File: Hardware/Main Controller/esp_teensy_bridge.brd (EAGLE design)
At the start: 102.8 x 87.9 mm, 42 parts, among them IC1 BQ79600PWRQ1, Q1 SI7611DN-T1-GE3, Q2 SI7611DN-T1-GE3, Q3 SI7611DN-T1-GE3, Q4 SI7611DN-T1-GE3

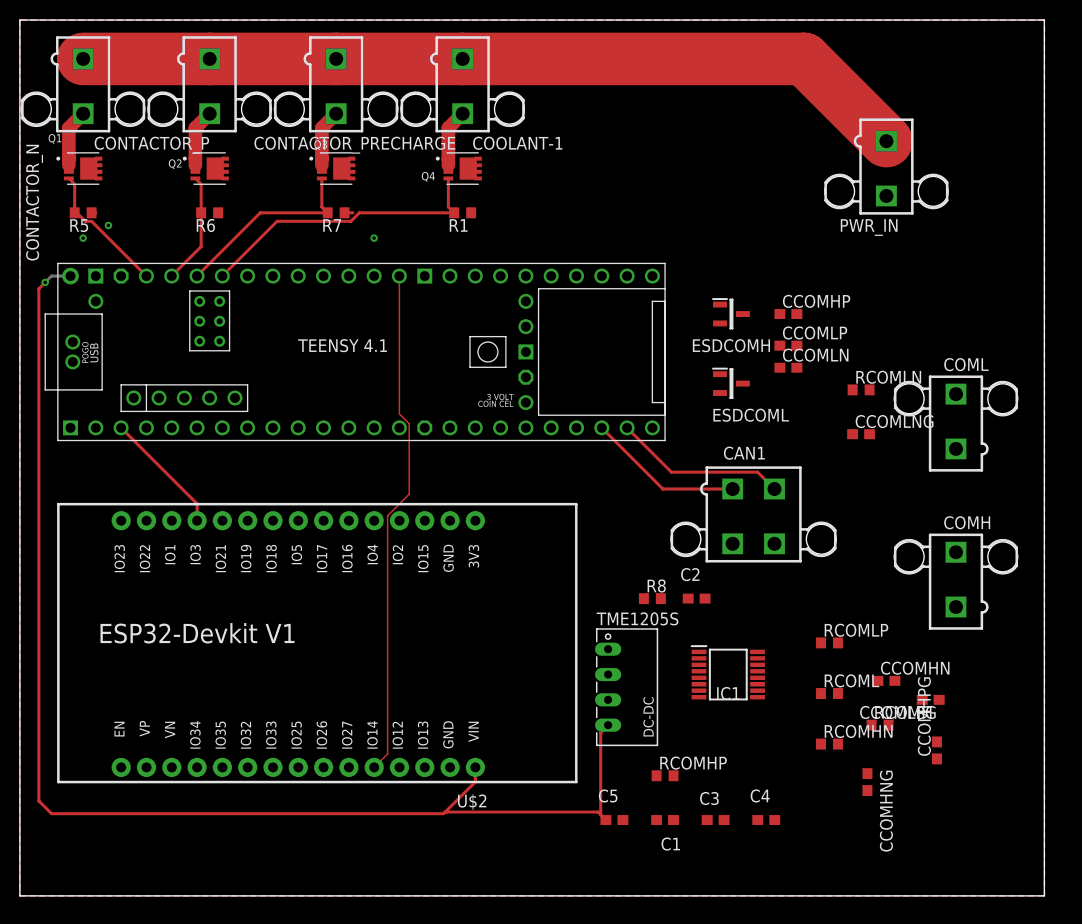
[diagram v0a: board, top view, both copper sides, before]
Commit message: connected some stuff
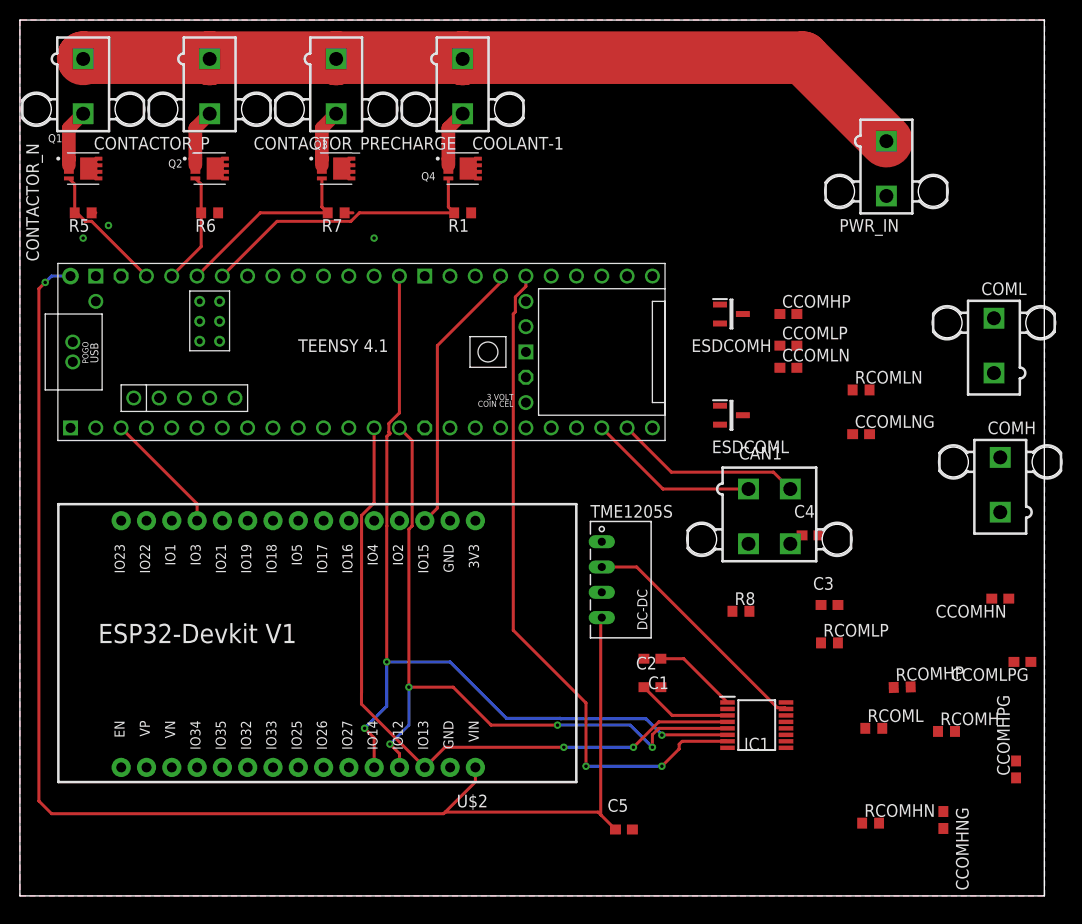
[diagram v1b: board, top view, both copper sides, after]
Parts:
- moved C4 28.9 mm to (79.4, 36.2)
- moved RCOMHP 25.4 mm to (88.6, 21.0), turned to 1.8 degrees
- moved C3 24.4 mm to (81.3, 29.2)
- moved C1 16.2 mm to (63.5, 23.8)
- moved CCOMHN 14.1 mm to (98.4, 29.8), turned to 180 degrees
- moved TME1205S 10.8 mm to (58.4, 31.8)
- moved COMH 10.5 mm to (98.4, 41.3)
- moved CCOMLPG 9.96 mm to (100.6, 23.5)
- moved C2 9.94 mm to (63.5, 21.0)
- moved R8 8.98 mm to (72.4, 28.6)
- moved RCOMHN 8.95 mm to (85.4, 7.30)
- moved COML 8.52 mm to (97.8, 55.2)
- moved CCOMHNG 8.52 mm to (92.7, 7.62)
- moved CCOMHPG 8.16 mm to (100.0, 12.7)
- moved RCOMH 6.70 mm to (93.0, 16.5)
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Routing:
- net MISO: track 0.00 -> 72.0 mm, vias 0 -> 4
- net MOSI: track 0.00 -> 69.5 mm, vias 0 -> 2
- net CS0: track 0.00 -> 68.3 mm, vias 0 -> 2
- net SCK: track 51.2 -> 88.7 mm, vias 0 -> 3
- net CS1: track 0.00 -> 27.7 mm
- net VCC: track 84.1 -> 109.0 mm
- net 5V: track 128.0 -> 139.9 mm
- net VIO: track 0.00 -> 9.56 mm
- net N$1: track 0.00 -> 8.51 mm
- net N$8: track 17.3 -> 18.9 mm
- net N$7: track 15.7 -> 17.3 mm
